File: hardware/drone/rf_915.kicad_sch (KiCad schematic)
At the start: 30 parts, among them U10 PE4259, U2 SX1262IMLTRT, U24 MM8030_2610RJ3, Y2 Crystal_GND24

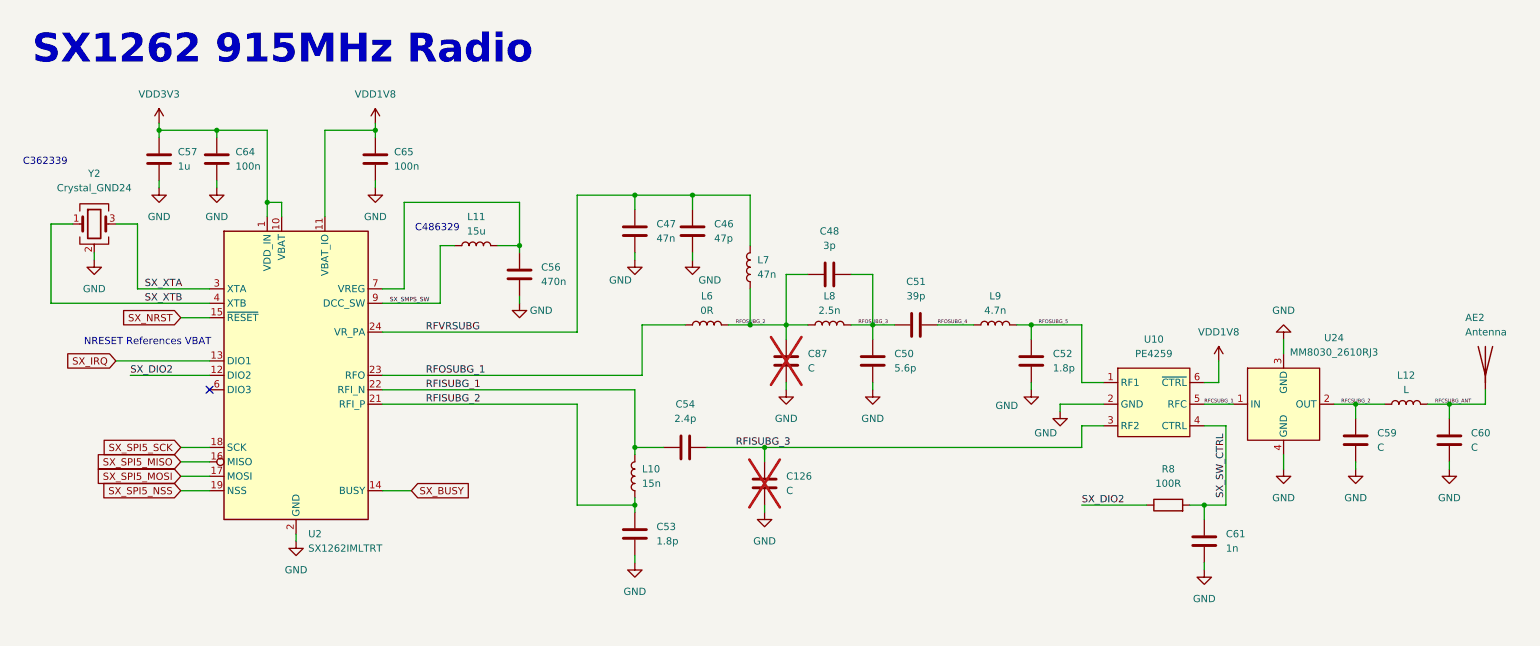
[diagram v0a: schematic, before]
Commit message: Small cleanup and more power routing
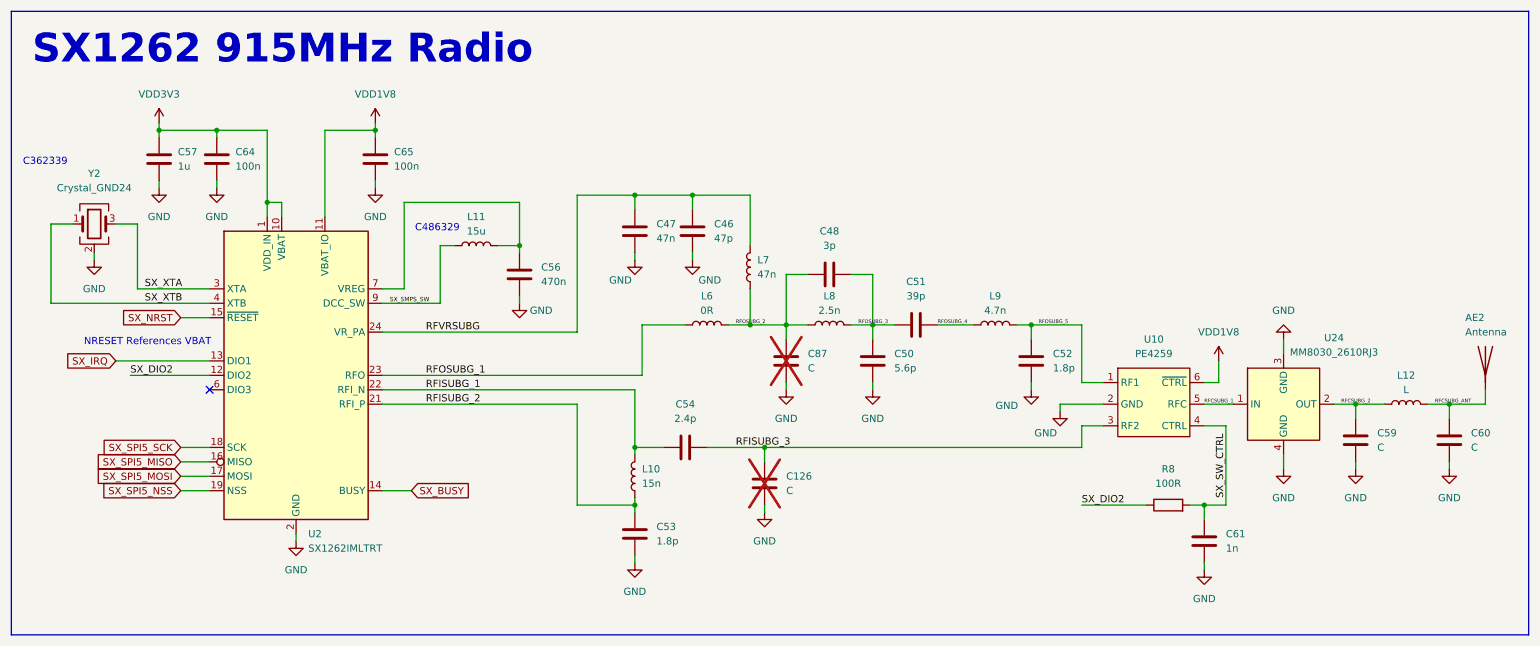
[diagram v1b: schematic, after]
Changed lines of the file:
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@@
 	(generator_version "10.0")
 	(paper "A4")
+	(rectangle
+		(start 14.605 17.145)
+		(end 281.94 127)
+		(stroke
+			(width 0)
+			(type default)
+		)
+		(fill
+			(type none)
+		)
+	)
 	(text "SX1262 915MHz Radio"
 		(exclude_from_sim no)
